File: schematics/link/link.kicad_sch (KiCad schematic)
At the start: 23 parts, among them J1 S2, J2 ARJM11C7-114-BA-EW2, J3 SDI12, J4 S1

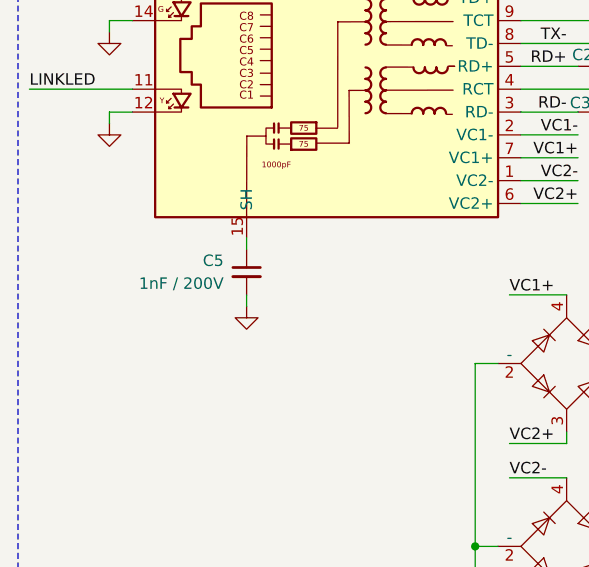
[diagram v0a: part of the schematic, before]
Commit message: fix: git history
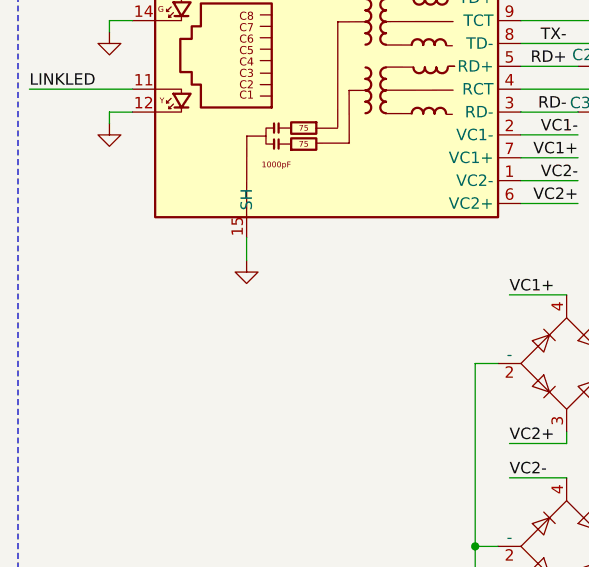
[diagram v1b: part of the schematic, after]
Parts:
- removed C5: 1nF / 200V, Capacitor_SMD:C_0402_1005Metric, symbol Device:C_Small
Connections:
- net GND: now also J2.15 (SH), J2.16 (SH)
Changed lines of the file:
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@@
 	(wire
 		(pts
-			(xy 50.8 140.97) (xy 50.8 142.24)
-		)
-		(stroke
-			(width 0)
-			(type default)
-		)
-	)
-	(wire
-		(pts
 			(xy 195.58 38.1) (xy 203.2 38.1)
 		)
@@
 	(wire
 		(pts
-			(xy 50.8 148.59) (xy 50.8 147.32)
+			(xy 50.8 140.97) (xy 50.8 143.51)
 		)
 		(stroke
@@
 	(symbol
 		(lib_id "power:GND")
-		(at 50.8 148.59 0)
+		(at 50.8 143.51 0)
 		(mirror y)
 		(unit 1)
@@
 		(dnp no)
 		(property "Reference" "#PWR017"
-			(at 50.8 154.94 0)
+			(at 50.8 149.86 0)
 			(hide yes)
 			(show_name no)
@@
 		)
 		(property "Value" "GND"
-			(at 50.8 152.4 0)
+			(at 50.8 147.32 0)
 			(hide yes)
 			(show_name no)
@@
 		)
 		(property "Footprint" ""
-			(at 50.8 148.59 0)
+			(at 50.8 143.51 0)
 			(hide yes)
 			(show_name no)
@@
 		)
 		(property "Datasheet" ""
-			(at 50.8 148.59 0)
+			(at 50.8 143.51 0)
 			(hide yes)
 			(show_name no)
@@
 		)
 		(property "Description" "Power symbol creates a global label with name \"GND\" , ground"
-			(at 50.8 148.59 0)
+			(at 50.8 143.51 0)
 			(hide yes)
 			(show_name no)
@@
 					(unit 1)
 				)
-			)
-		)
-	)
-	(symbol
-		(lib_id "Device:C_Small")
-		(at 50.8 144.78 0)
-		(mirror y)
-		(unit 1)
-		(body_style 1)
-		(exclude_from_sim no)
-		(in_bom yes)
-		(on_board yes)
-		(in_pos_files yes)
-		(dnp no)
-		(fields_autoplaced yes)
-		(property "Reference" "C5"
-			(at 48.26 143.5162 0)
-			(show_name no)
-			(do_not_autoplace no)
-			(effects
-				(font
-					(size 1.27 1.27)
-				)
-				(justify left)
-			)
-		)
-		(property "Value" "1nF / 200V"
-			(at 48.26 146.0562 0)
-			(show_name no)
-			(do_not_autoplace no)
-			(effects
-				(font
-					(size 1.27 1.27)
-				)
-				(justify left)
-			)
-		)
-		(property "Footprint" "Capacitor_SMD:C_0402_1005Metric"
-			(at 50.8 144.78 0)
-			(hide yes)
-			(show_name no)
-			(do_not_autoplace no)
-			(effects
-				(font
-					(size 1.27 1.27)
-				)
-			)
-		)
-		(property "Datasheet" ""
-			(at 50.8 144.78 0)
-			(hide yes)
-			(show_name no)
-			(do_not_autoplace no)
-			(effects
-				(font
-					(size 1.27 1.27)
-				)
-			)
-		)
-		(property "Description" "Unpolarized capacitor, small symbol"
-			(at 50.8 144.78 0)
-			(hide yes)
-			(show_name no)
-			(do_not_autoplace no)
-			(effects
-				(font
-					(size 1.27 1.27)
-				)
-			)
-		)
-		(property "FT Rotation Offset" ""
-			(at 50.8 144.78 0)
-			(hide yes)
-			(show_name no)
-			(do_not_autoplace no)
-			(effects
-				(font
-					(size 1.27 1.27)
-				)
-			)
-		)
-		(property "LCSC" "C1588 "
-			(at 50.8 144.78 0)
-			(hide yes)
-			(show_name no)
-			(do_not_autoplace no)
-			(effects
-				(font
-					(size 1.27 1.27)
-				)
-			)
-		)
-		(pin "1"
-		)
-		(pin "2"
-		)
-		(instances
-			(project "link"
-				(path "/e6a73b1b-9233-47b9-8d6b-253608bed688"
-					(reference "C5")
-					(unit 1)
-				)
